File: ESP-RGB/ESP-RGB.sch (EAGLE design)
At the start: 1 part, among them IC1 ESP-12E/F

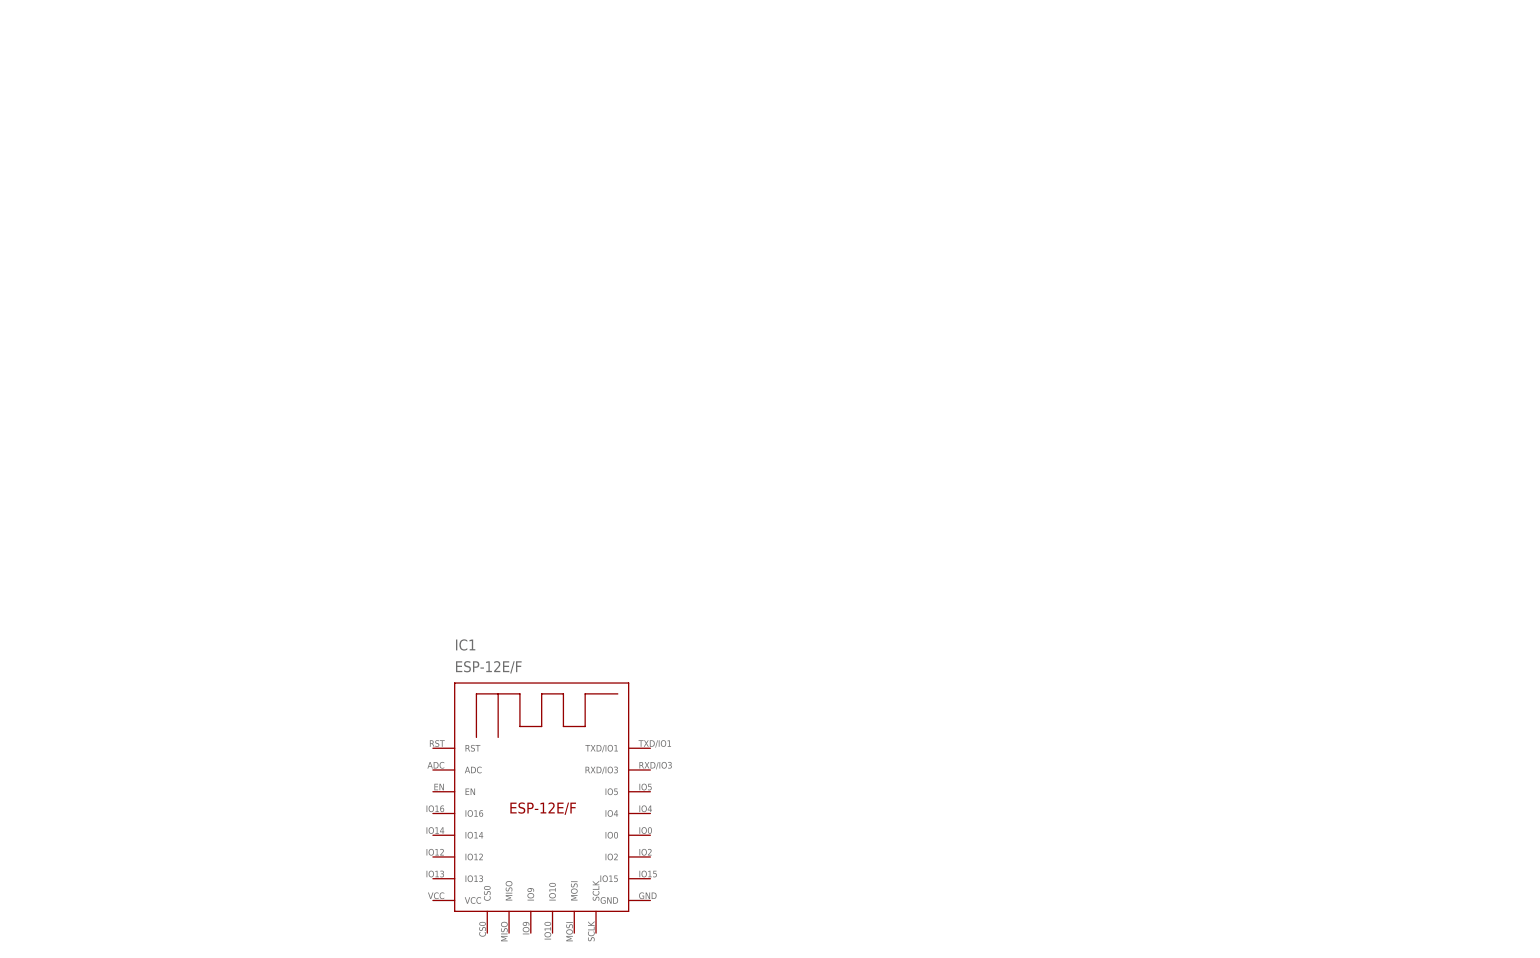
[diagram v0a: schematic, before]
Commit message: some schematic
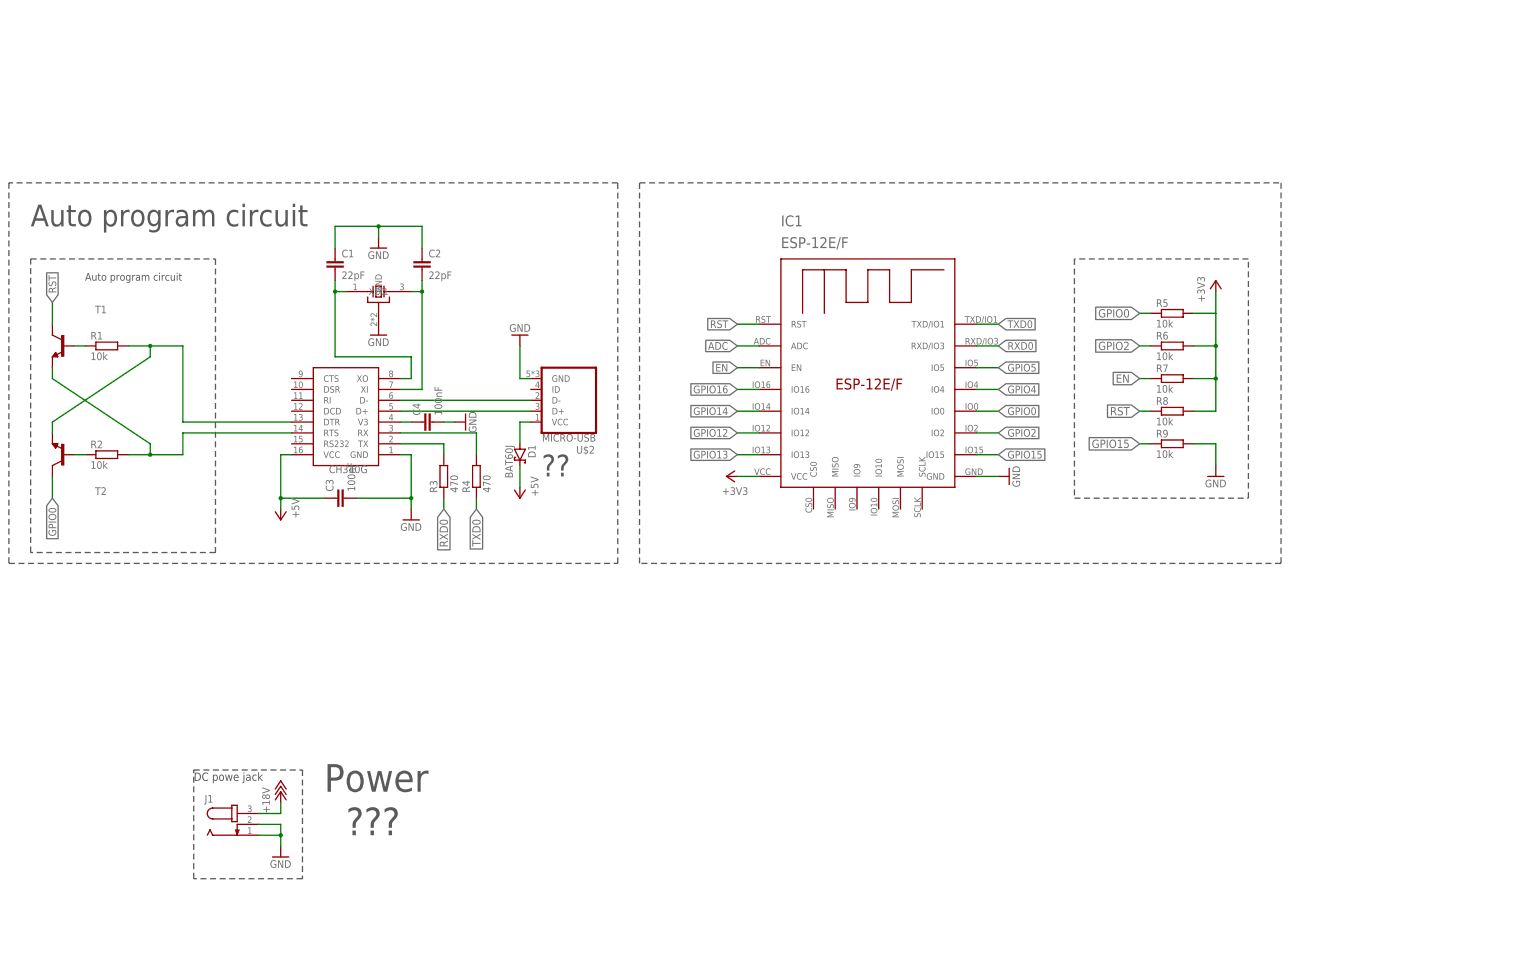
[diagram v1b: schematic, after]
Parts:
- added C1, C2: 22pF, rcl:C-EUC0805K
- added C3, C4: 100nF, rcl:C-EUC0805K
- added D1: BAT60J, diode:BAT60J
- added J1: (no value), con-jack:JACK-PLUG0
- added R1, R2, R5, R6, R7, R8, R9: 10k, rcl:R-EU_R0603
- added R3, R4: 470, rcl:R-EU_R0603
- added T1, T2: (no value), transistor:BC817-16-NPN-SOT23-BEC
- added U$1: CH340G, ESP-RGB:CH340G
- added U$2: MICRO-USB, ESP-RGB:MICRO-USB
- added U$3: CTS_32X25_SMD, ESP-RGB:CTS_32X25_SMD
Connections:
- new net +18V: J1.3
- new net +3V3: IC1.VCC, R5.2, R6.2, R7.2, R8.2
- new net +5V: C3.1, D1.C, U$1.VCC
- new net ADC: IC1.ADC
- new net EN: IC1.EN, R7.1
- new net GND: C1.1, C2.1, C3.2, C4.2, IC1.GND, J1.1, J1.2, R9.2, U$1.GND, U$2.GND, U$3.GND
- new net GPIO0: IC1.IO0, R5.1, T2.C
- new net GPIO12: IC1.IO12
- new net GPIO13: IC1.IO13
- new net GPIO14: IC1.IO14
- new net GPIO15: IC1.IO15, R9.1
- new net GPIO16: IC1.IO16
- new net GPIO2: IC1.IO2, R6.1
- new net GPIO4: IC1.IO4
- new net GPIO5: IC1.IO5
- new net N$1: R2.2, T1.E, U$1.RTS
- new net N$10: C1.2, U$1.XO, U$3.X1
- new net N$11: C2.2, U$1.XI, U$3.X2
- new net N$12: R4.2, U$1.RX
- new net N$13: C4.1, U$1.V3
- new net N$2: R1.2, T2.E, U$1.DTR
- new net N$3: R1.1, T1.B
- new net N$4: R2.1, T2.B
- new net N$5: U$1.D-, U$2.D-
- new net N$6: U$1.D+, U$2.D+
- new net N$7: D1.A, U$2.VCC
- new net N$9: R3.2, U$1.TX
- new net RST: IC1.RST, R8.1, T1.C
- new net RXD0: IC1.RXD/IO3, R3.1
- new net TXD0: IC1.TXD/IO1, R4.1
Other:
- note added: "??"
- note added: "???"
- note added: "Auto program circuit"
- note added: "DC powe jack"
- note added: "Power"
- moved on the sheet: IC1

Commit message: add power module
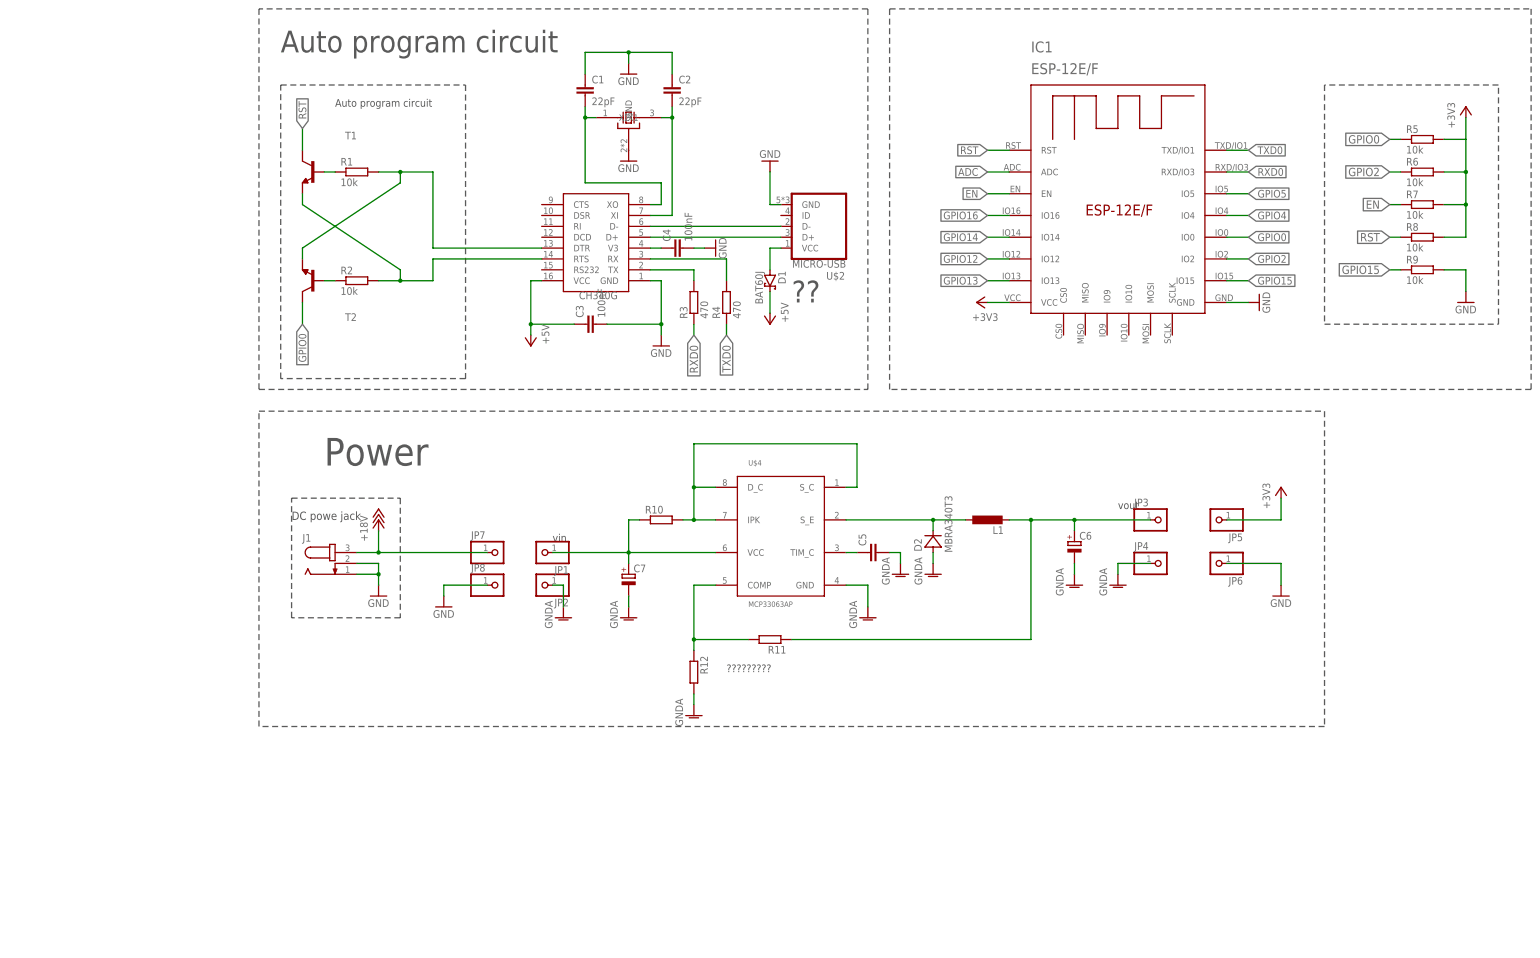
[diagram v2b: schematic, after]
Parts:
- added C5: (no value), rcl:C-EUC0805K
- added C6, C7: (no value), rcl:CPOL-EU153CLV-0505
- added D2: MBRA340T3, diode:MBRA340T3
- added JP1, JP2, JP3, JP4, JP5, JP6, JP7, JP8: (no value), pinhead:PINHD-1X1
- added L1: (no value), rcl:L-EUPIS2816
- added R10: (no value), rcl:R-EU_R1206W
- added R11, R12: (no value), rcl:R-EU_R0603
- added U$4: MCP33063AP, ESP-RGB:MCP33063AP
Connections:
- new net GNDA: C5.2, C6.-, C7.-, D2.A, JP2.1, JP4.1, R12.2, U$4.GND
- new net N$15: R11.2, R12.1, U$4.COMP
- new net N$16: R10.2, U$4.D_C, U$4.IPK, U$4.S_C
- new net N$17: D2.C, L1.1, U$4.S_E
- new net N$19: C5.1, U$4.TIM_C
- new net N$21: C6.+, JP3.1, L1.2, R11.1
- new net N$8: C7.+, JP1.1, R10.1, U$4.VCC
- net +18V: now also JP7.1
- net +3V3: now also JP5.1
- net GND: now also JP6.1, JP8.1
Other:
- note added: "?????????"
- note added: "vin"
- note added: "vout"
- note removed: "???"
- moved on the sheet: C1, C2, C3, C4, D1, IC1, J1, R1, R2, R3, R4, R5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
